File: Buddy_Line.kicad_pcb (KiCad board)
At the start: 2 copper layers, 65 x 25 mm, 18 parts, among them J1 AudioJack3, J2 Conn_01x04_Pin, U3 TPA6110A2DGN

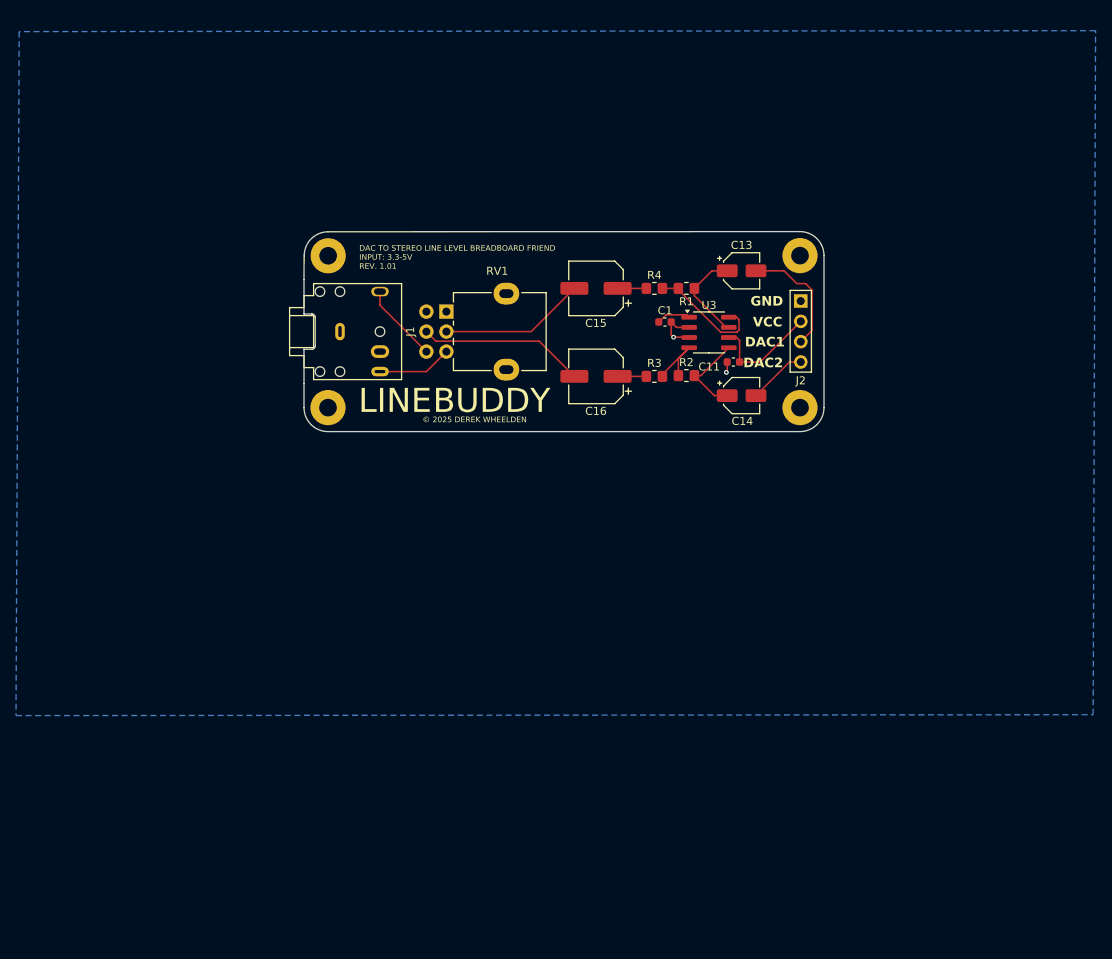
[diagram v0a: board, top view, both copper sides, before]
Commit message: New form factor
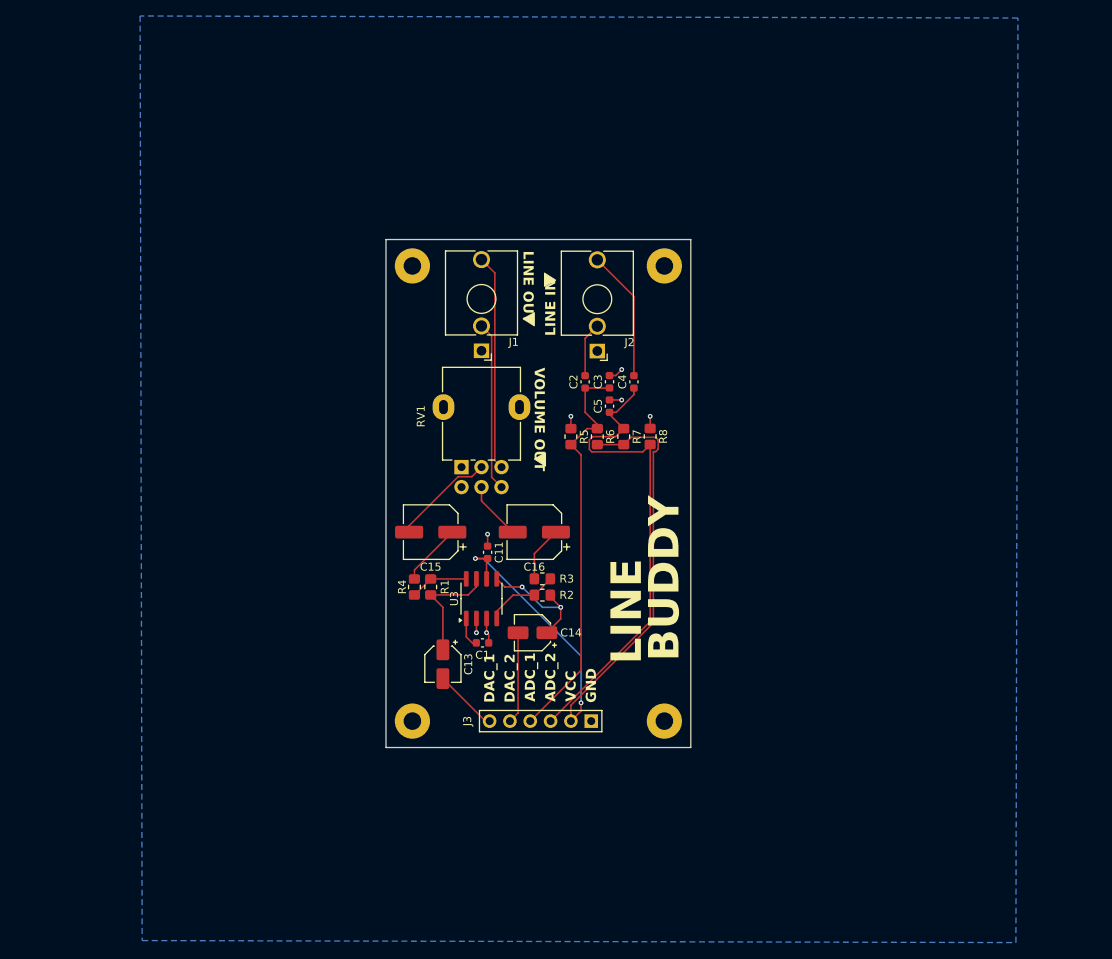
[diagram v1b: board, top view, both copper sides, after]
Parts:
- added C2: 10u, Capacitor_SMD:C_0603_1608Metric, F.Cu at (145.5, 90.2)
- added C3: 0.1u, Capacitor_SMD:C_0603_1608Metric, F.Cu at (148.6, 90.2)
- added C4: 10u, Capacitor_SMD:C_0603_1608Metric, F.Cu at (151.6, 90.2)
- added C5: 0.1u, Capacitor_SMD:C_0603_1608Metric, F.Cu at (148.6, 93.2)
- added J3: Conn_01x06_Pin, Connector_PinSocket_2.54mm:PinSocket_1x06_P2.54mm_Vertical, F.Cu at (133.6, 132.6)
- added R5: 1K, Resistor_SMD:R_0805_2012Metric_Pad1.20x1.40mm_HandSolder, F.Cu at (143.8, 97.0)
- added R6: 1K, Resistor_SMD:R_0805_2012Metric_Pad1.20x1.40mm_HandSolder, F.Cu at (147.1, 97.0)
- added R7: 1K, Resistor_SMD:R_0805_2012Metric_Pad1.20x1.40mm_HandSolder, F.Cu at (150.4, 97.0)
- added R8: 1K, Resistor_SMD:R_0805_2012Metric_Pad1.20x1.40mm_HandSolder, F.Cu at (153.7, 97.0)
- J1: footprint Connector_Audio:Jack_3.5mm_CUI_SJ1-3524N_Horizontal -> Connector_Audio:Jack_3.5mm_QingPu_WQP-PJ398SM_Vertical_CircularHoles
- J2: value Conn_01x04_Pin -> AudioJack3; footprint Connector_PinHeader_2.54mm:PinHeader_1x04_P2.54mm_Vertical -> Connector_Audio:Jack_3.5mm_QingPu_WQP-PJ398SM_Vertical_CircularHoles
- moved H1 71.8 mm to (155.4, 132.6)
- moved C13 61.7 mm to (127.8, 125.5), turned to -90 degrees
- moved H4 51.6 mm to (124.0, 75.7)
- moved R1 49.1 mm to (126.2, 115.8), turned to 90 degrees
- moved R4 47.9 mm to (124.2, 115.8), turned to -90 degrees
- moved C1 46.1 mm to (132.7, 122.8)
- moved U3 43.8 mm to (132.6, 117.3), turned to 90 degrees
- moved H2 40.6 mm to (124.0, 132.6)
- moved C14 39.5 mm to (139.0, 121.5), turned to 180 degrees
- moved C11 38.9 mm to (133.3, 111.5), turned to -90 degrees
- moved C15 36.8 mm to (126.2, 109.0)
- moved R2 32.8 mm to (140.2, 116.8)
- moved R3 28.9 mm to (140.2, 114.8)
- moved J2 25.5 mm to (147.1, 86.3)
- moved C16 20.9 mm to (139.2, 109.0)
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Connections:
- C13 pad 2: unconnected-(J2-Pin_2-Pad2) -> DAC_1
- C14 pad 2: unconnected-(J2-Pin_1-Pad1) -> DAC_2
- J1 pad TN: GND -> Net-(J1-PadTN)
- RV1 pad 6: Net-(J1-PadR) -> Net-(J1-PadTN)
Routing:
- net +3.3V: track 13.9 -> 79.0 mm, vias 0 -> 2
- net ADC_2: track 0.00 -> 61.5 mm
- net ADC_1: track 0.00 -> 50.6 mm
- net Net-(J1-PadTN): track 0.00 -> 21.2 mm
- net Net-(J1-PadT): track 9.34 -> 27.0 mm
- net Net-(C4-Pad2): track 0.00 -> 16.4 mm
- net unconnected-(J2-Pin_2-Pad2): track 15.0 -> 0.00 mm
- net unconnected-(RV1-Pad5): track 20.8 -> 7.25 mm
- net DAC_2: track 0.00 -> 11.5 mm
- net Net-(J1-PadR): track 9.90 -> 0.00 mm
- net DAC_1: track 0.00 -> 8.04 mm
- net Net-(R1-Pad2): track 14.8 -> 7.31 mm
- net unconnected-(J2-Pin_1-Pad1): track 7.34 -> 0.00 mm
- net Net-(C2-Pad2): track 0.00 -> 6.81 mm
- net unconnected-(RV1-Pad2): track 18.2 -> 12.9 mm
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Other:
- board size 65 x 25 mm -> 38.1 x 63.5 mm
- board text added: "${REFERENCE}"
- board text added: "ADC_1"
- board text added: "ADC_2"
- board text added: "DAC_1"
- board text added: "DAC_2"
- board text added: "LINE IN"
- board text added: "LINE OUT"
- board text added: "VOLUME OUT"
- board text removed: "DAC TO STEREO LINE LEVEL BREADBOARD FRIEND INPUT: 3.3-5V REV. 1.01"
- board text removed: "DAC1"
- board text removed: "DAC2"
- board text removed: "© 2025 DEREK WHEELDEN"
